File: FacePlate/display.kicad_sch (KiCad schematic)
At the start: 16 parts, among them U1 GC9A, U2 GC9A

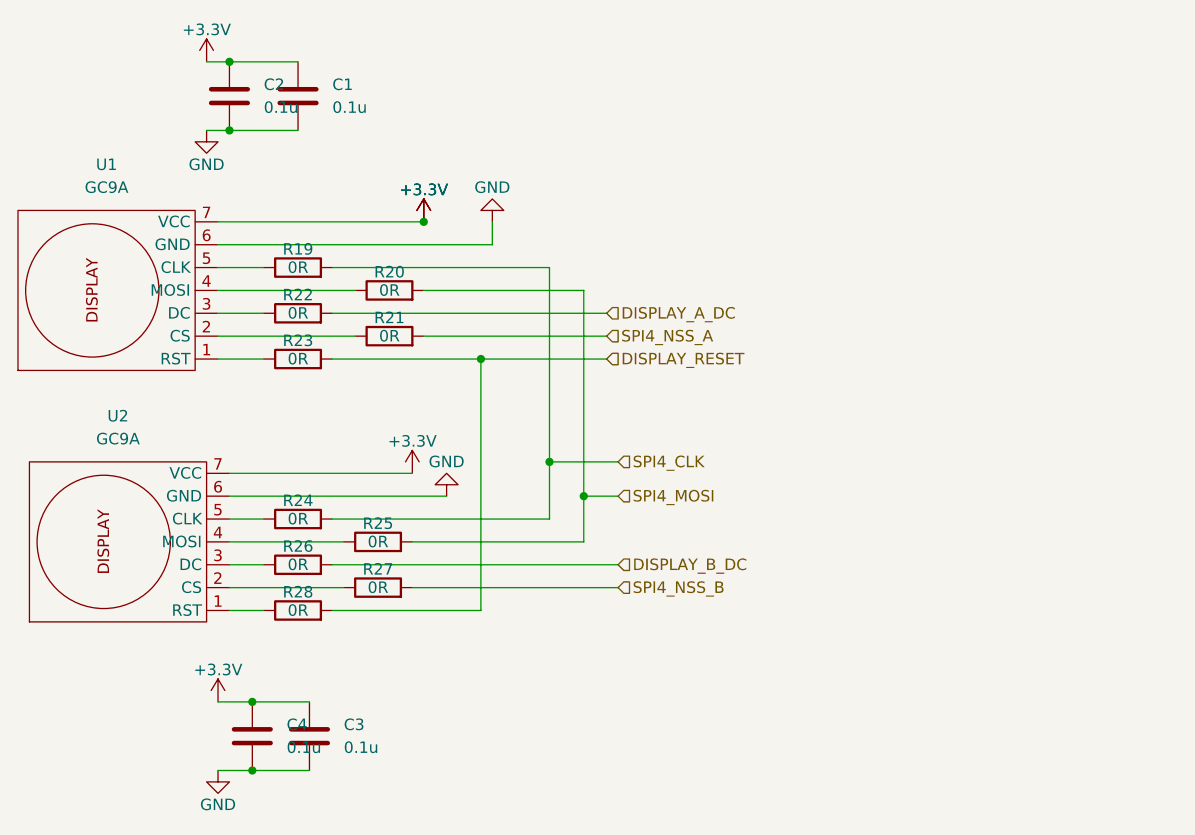
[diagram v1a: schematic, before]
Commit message: production + fixing libraries
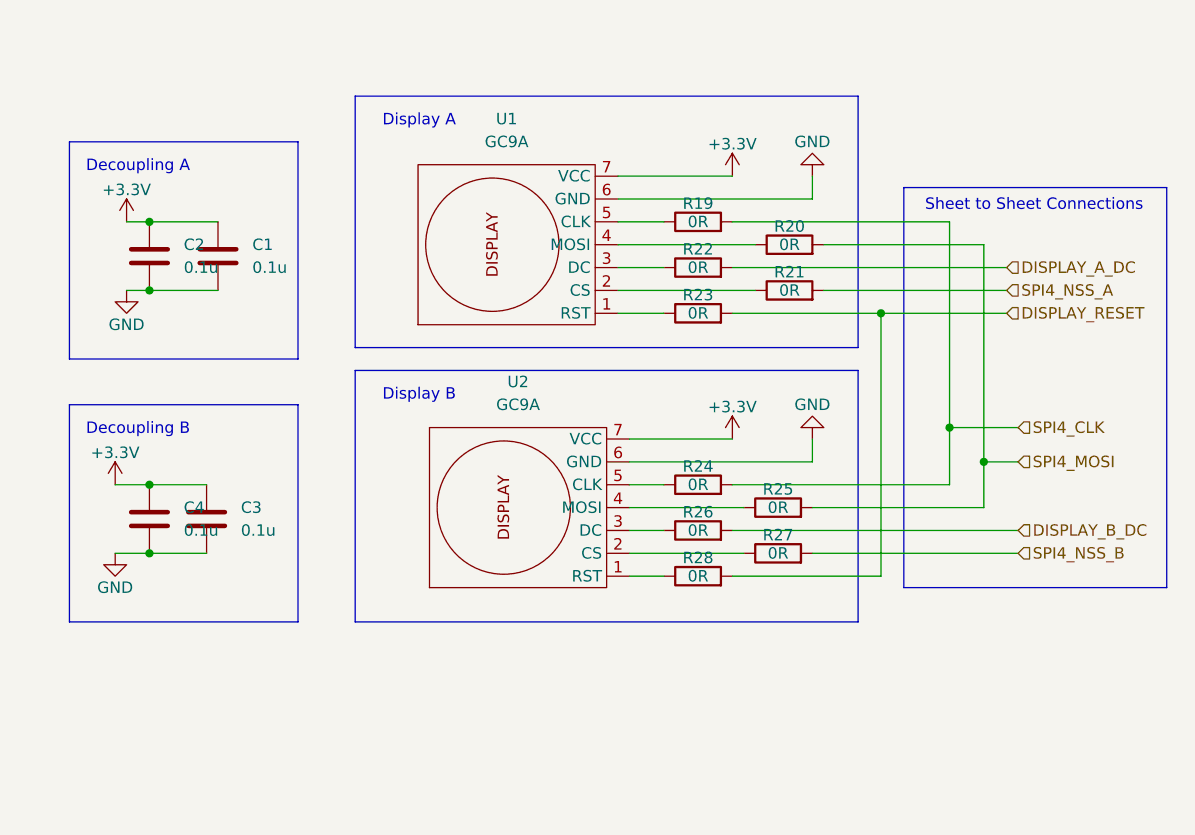
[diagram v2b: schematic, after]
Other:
- note added: "Decoupling A"
- note added: "Decoupling B"
- note added: "Display A"
- note added: "Display B"
- note added: "Sheet to Sheet Connections"
- moved on the sheet: C1, C2, C3, C4, R19, R20, R21, R22, R23, R24, R25, R26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
